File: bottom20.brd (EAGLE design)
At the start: 160 x 140 mm, 142 parts, among them T1:IC1 MULTIPLEXER, T1:R1 20k, T1:R10 20k, T1:R11 20k, T1:R12 20k, T1:R13 20k, T1:R14 20k, T1:R15 20k, T1:R16 20k, T1:R17 10k, T1:R2 20k, T1:R3 20k, T1:R4 20k, T1:R5 20k, T1:R6 20k, T1:R7 20k, T1:R8 20k, T1:R9 20k, T1:T1 SFH320, T1:T10 SFH320, T1:T11 SFH320, T1:T12 SFH320, T1:T13 SFH320, T1:T14 SFH320, T1:T15 SFH320, T1:T16 SFH320, T1:T2 SFH320, T1:T3 SFH320, T1:T4 SFH320, T1:T5 SFH320, T1:T6 SFH320, T1:T7 SFH320, T1:T8 SFH320, T1:T9 SFH320, T2:IC1 MULTIPLEXER, T2:R1 20k, T2:R10 20k, T2:R11 20k, T2:R12 20k, T2:R13 20k, T2:R14 20k, T2:R15 20k, T2:R16 20k, T2:R17 10k, T2:R2 20k, T2:R3 20k, T2:R4 20k, T2:R5 20k, T2:R6 20k, T2:R7 20k, T2:R8 20k, T2:R9 20k, T2:T1 SFH320, T2:T10 SFH320, T2:T11 SFH320, T2:T12 SFH320, T2:T13 SFH320, T2:T14 SFH320, T2:T15 SFH320, T2:T16 SFH320, T2:T2 SFH320, T2:T3 SFH320, T2:T4 SFH320, T2:T5 SFH320, T2:T6 SFH320, T2:T7 SFH320, T2:T8 SFH320, T2:T9 SFH320

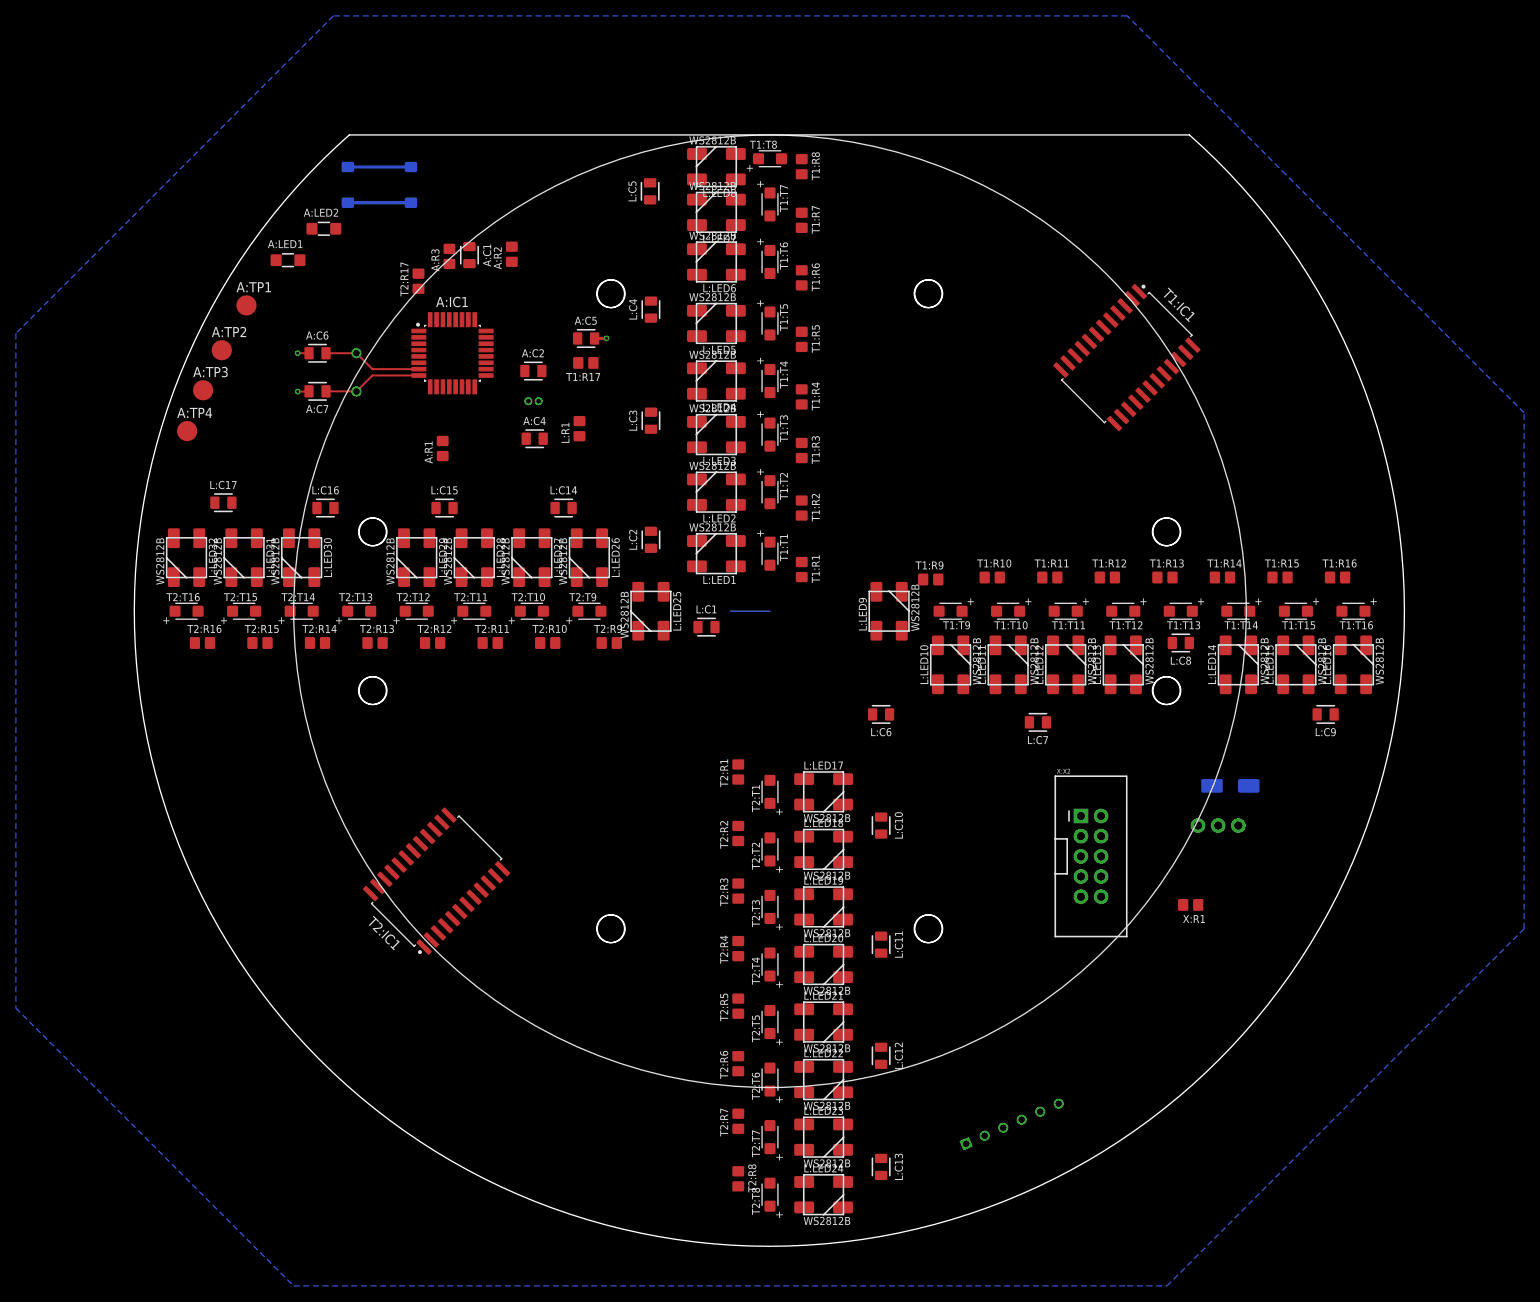
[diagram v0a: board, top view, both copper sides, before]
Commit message: - bot.brd/sch (begin of routing)
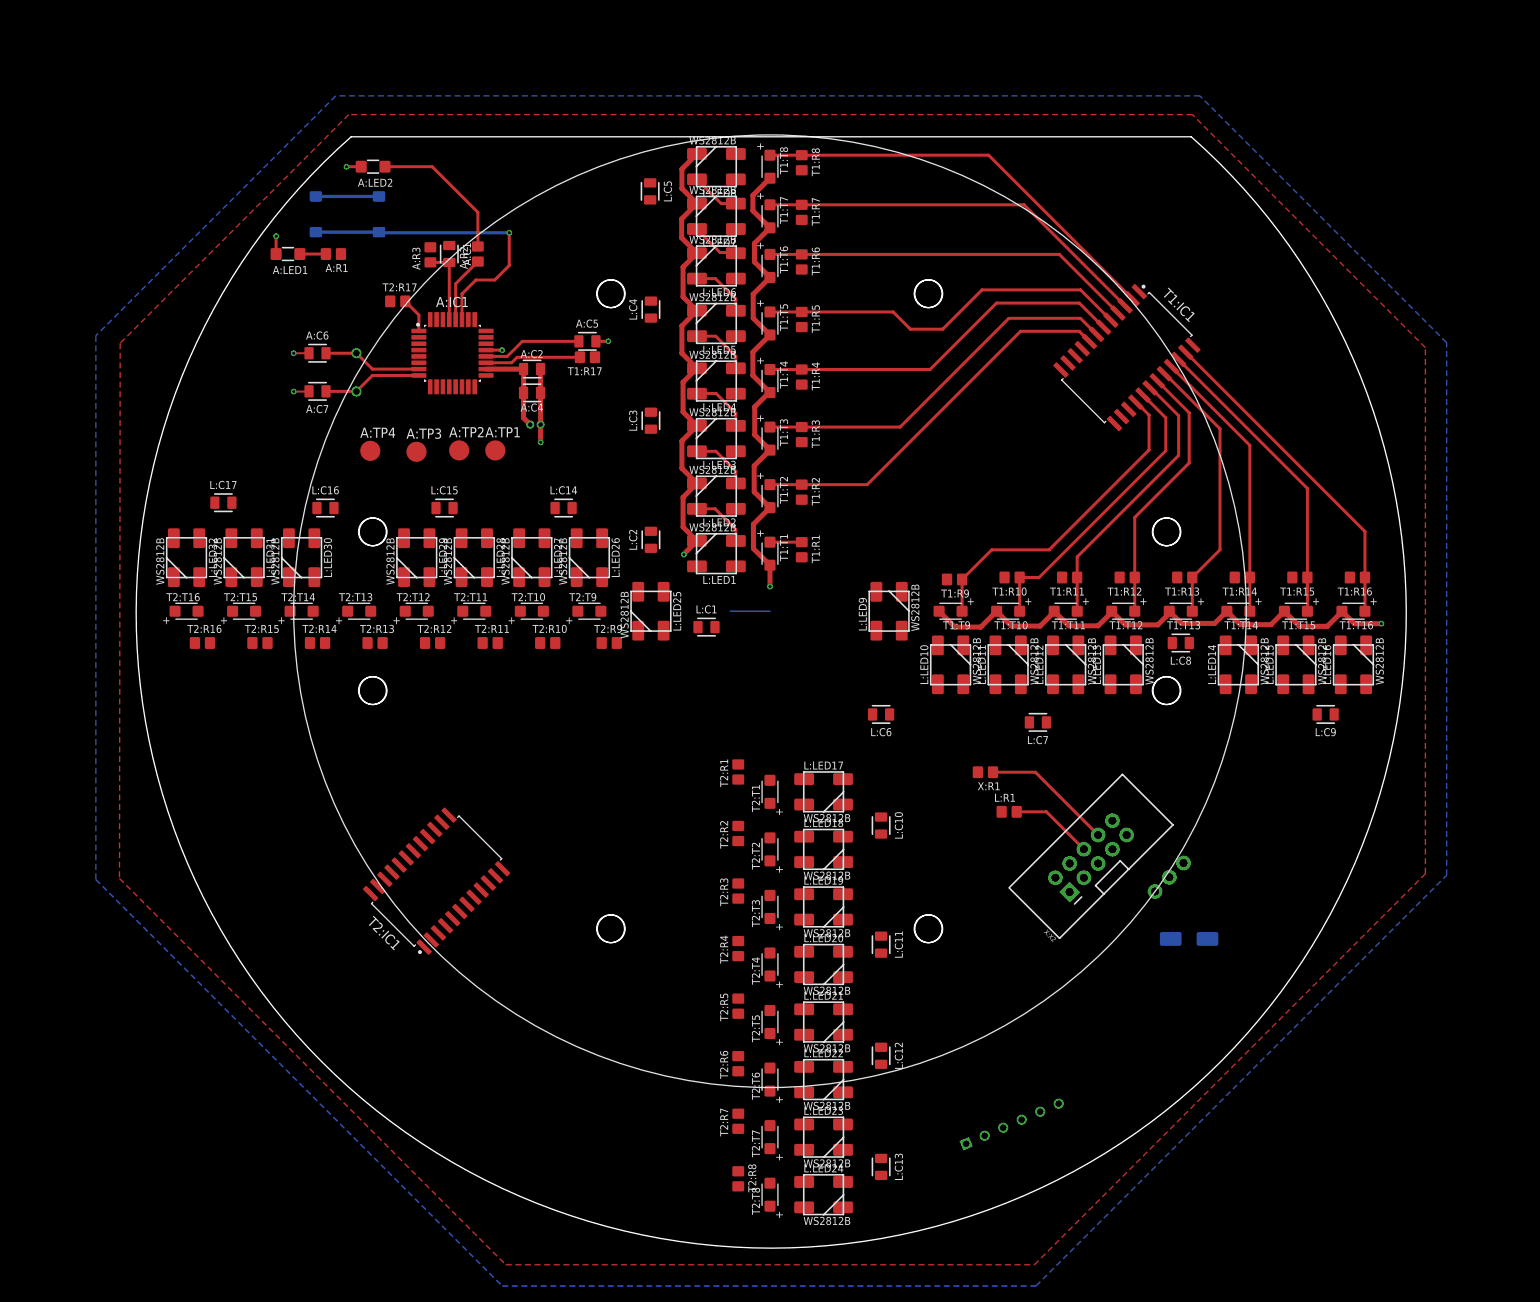
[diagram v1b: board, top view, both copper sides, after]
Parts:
- moved L:R1 72.5 mm to (30.1, -25.3), turned to 0 degrees
- moved A:TP1 36.3 mm to (-34.6, 20.3)
- moved A:TP2 32.5 mm to (-39.2, 20.3)
- moved X:R1 30.8 mm to (27.1, -20.3)
- moved A:R1 28.1 mm to (-55.0, 45.0), turned to 180 degrees
- moved A:TP3 28.0 mm to (-44.5, 20.1)
- moved A:TP4 23.2 mm to (-50.4, 20.2)
- moved X:D1 20.0 mm to (52.8, -41.3), turned to 180 degrees
- moved A:LED2 9.98 mm to (-50.0, 56.0), turned to 180 degrees
- moved P:X3 8.36 mm to (52.1, -31.7), turned to 315 degrees
- moved A:C4 5.79 mm to (-30.0, 27.5)
- moved A:S2 5.48 mm to (-53.2, 50.0)
- moved A:R2 4.28 mm to (-36.8, 45.0)
- moved T2:R17 3.64 mm to (-46.9, 39.0), turned to 0 degrees
- moved T1:R9 3.00 mm to (23.2, 4.00), turned to 180 degrees
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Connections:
- net N$1 renamed X:+12V
- removed net X:LED-IN: X:X2.6
- new net X:+5V: X:D1.1
- net +5V: no longer X:D1.1
- net LED-IN: now also X:X2.6
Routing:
- net GND: track 12.3 -> 221.6 mm, vias 3 -> 10
- net T1:N$9: track 0.00 -> 53.1 mm
- net T1:N$10: track 0.00 -> 50.0 mm
- net T1:N$2: track 0.00 -> 48.8 mm
- net T1:N$3: track 0.00 -> 47.7 mm
- net T1:N$5: track 0.00 -> 47.5 mm
- net T1:N$11: track 0.00 -> 46.9 mm
- net T1:N$4: track 0.00 -> 46.0 mm
- net T1:N$25: track 0.00 -> 42.0 mm
- net T1:N$7: track 0.00 -> 41.0 mm
- net T1:N$22: track 0.00 -> 37.9 mm
- net T1:N$12: track 0.00 -> 37.5 mm
- net T1:N$14: track 0.00 -> 35.4 mm
- net T1:N$20: track 0.00 -> 34.4 mm
- net T1:N$18: track 0.00 -> 34.3 mm
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- added copper zone on layer 1, net +5V

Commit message: - bot.brd (Routing)
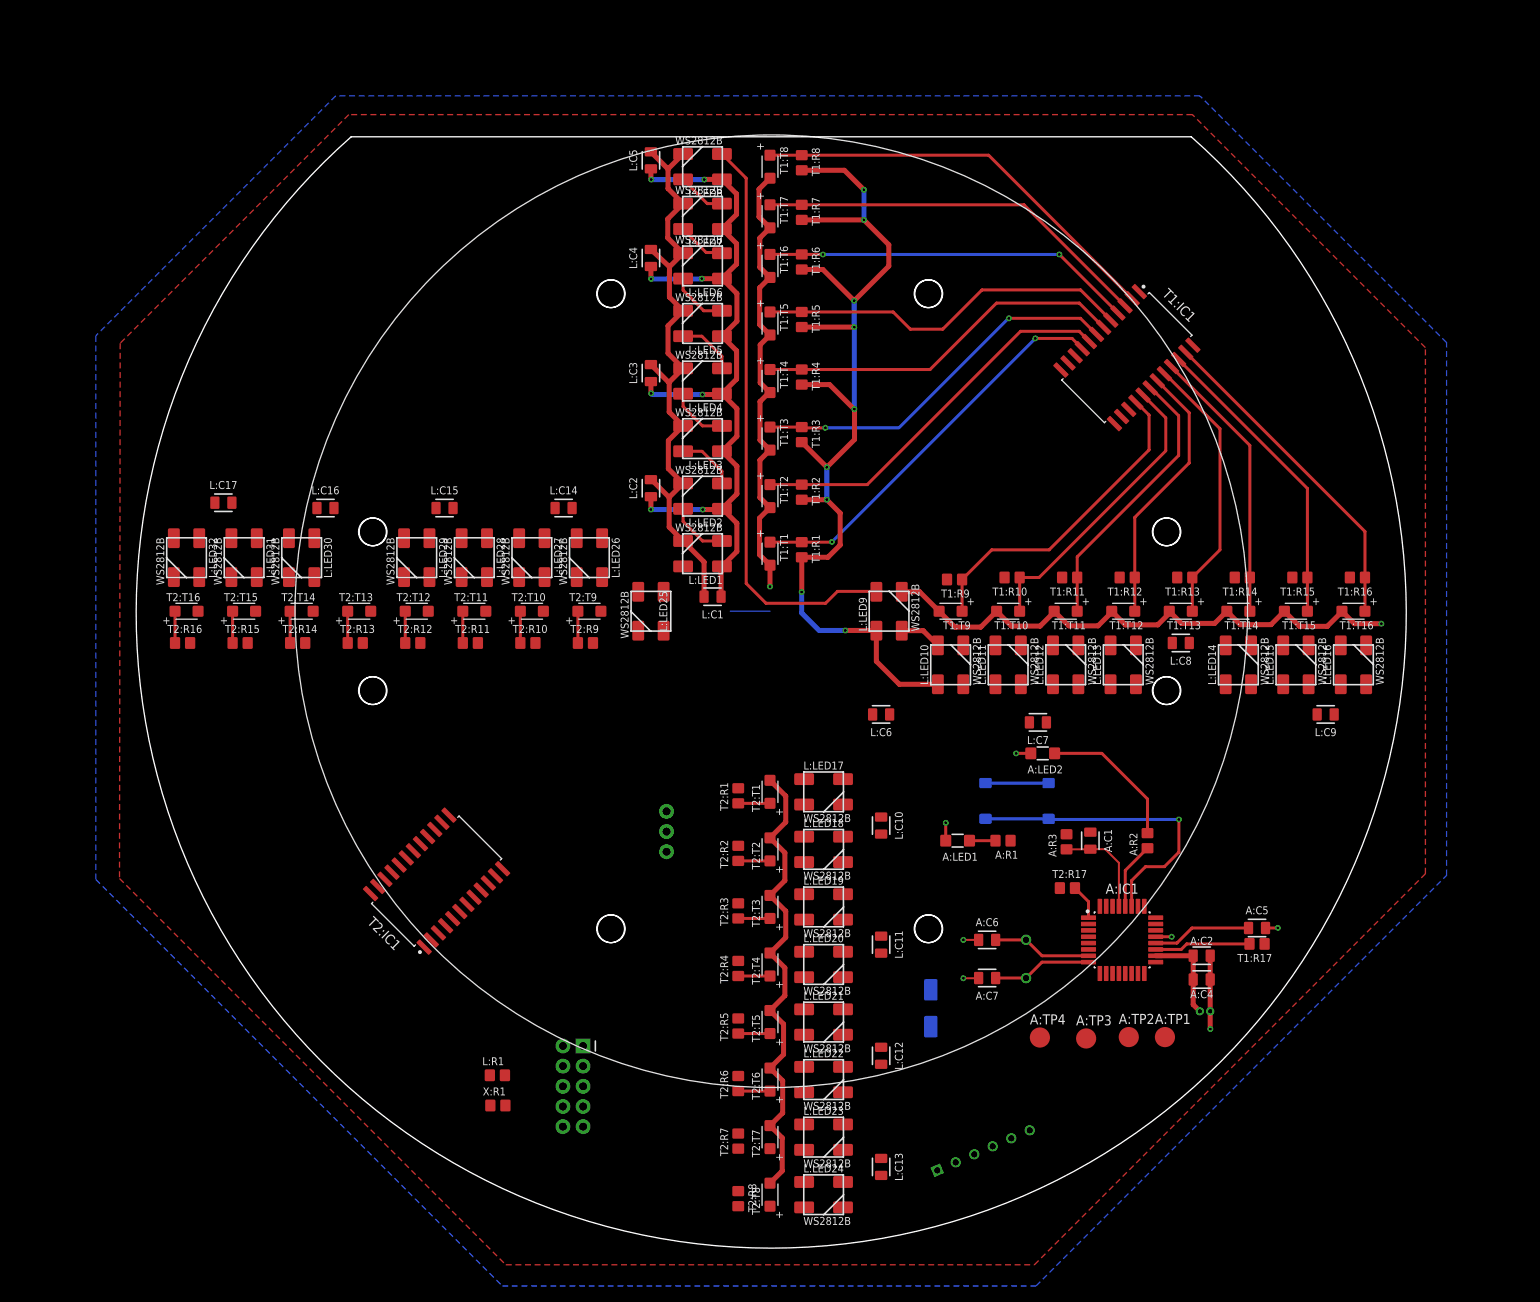
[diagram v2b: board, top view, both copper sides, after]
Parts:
- moved A:C2 112.1 mm to (54.4, -43.4)
- moved A:C3 112.1 mm to (54.8, -50.4)
- moved A:C4 112.1 mm to (54.4, -46.4)
- moved A:C5 112.1 mm to (61.4, -39.9)
- moved A:C6 112.1 mm to (27.4, -41.4)
- moved A:C7 112.1 mm to (27.4, -46.2)
- moved A:IC1 112.1 mm to (44.4, -41.4)
- moved A:LED1 112.1 mm to (23.6, -28.9)
- moved A:LED2 112.1 mm to (34.4, -17.9)
- moved A:Q1 112.1 mm to (32.3, -43.8)
- moved A:R1 112.1 mm to (29.4, -28.9)
- moved A:R2 112.1 mm to (47.6, -28.9)
- moved A:S2 112.1 mm to (31.1, -23.9)
- moved A:TP1 112.1 mm to (49.8, -53.6)
- moved A:TP2 112.1 mm to (45.2, -53.6)
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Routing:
- net +5V: track 12.1 -> 250.3 mm, vias 0 -> 17
- net GND: track 221.6 -> 302.5 mm, vias 10 -> 9
- net L:CON-1: track 0.00 -> 73.4 mm
- net T1:N$1: track 4.00 -> 50.5 mm, vias 0 -> 2
- net X:N$1: track 16.5 -> 0.00 mm
- net LED-IN: track 10.4 -> 0.00 mm
- net L:N$9: track 0.00 -> 5.32 mm
- net T2:N$7: track 0.00 -> 4.00 mm
- net T2:N$5: track 0.00 -> 4.00 mm
- net T2:N$4: track 0.00 -> 4.00 mm
- net T2:N$3: track 0.00 -> 4.00 mm
- net T2:N$26: track 0.00 -> 4.00 mm
- net T2:N$25: track 0.00 -> 4.00 mm
- net T2:N$22: track 0.00 -> 4.00 mm
- net T2:N$20: track 0.00 -> 4.00 mm
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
